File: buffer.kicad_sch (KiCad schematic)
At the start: 3 parts, among them U1 TL072

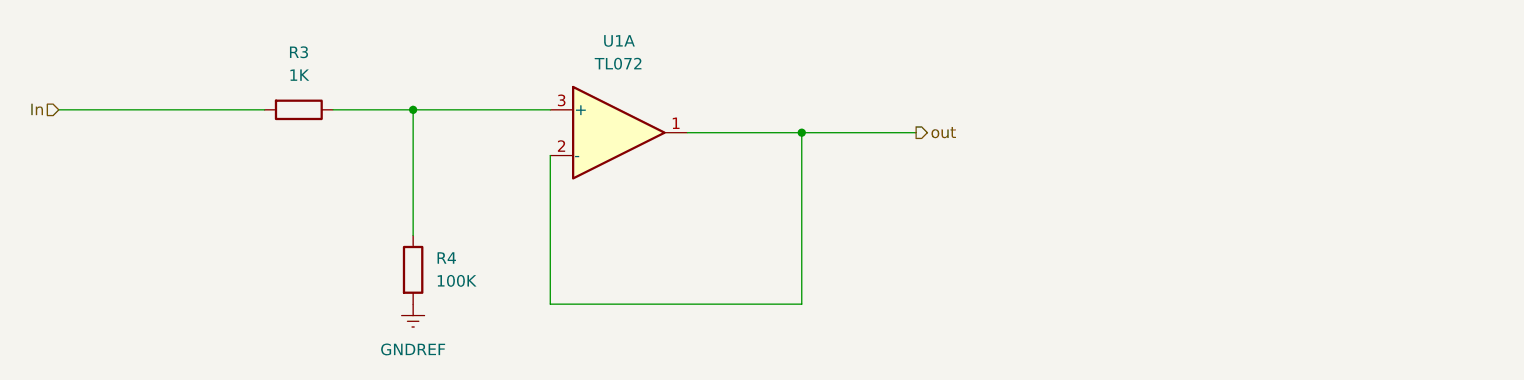
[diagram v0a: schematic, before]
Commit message: Fix input section
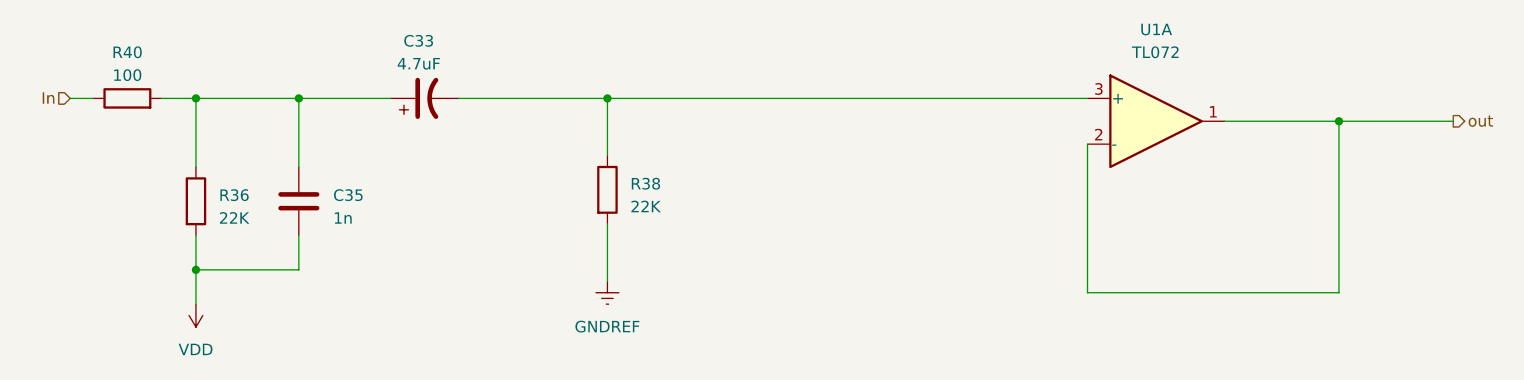
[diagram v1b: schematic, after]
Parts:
- removed R3: 1K, Resistor_THT:R_Axial_DIN0207_L6.3mm_D2.5mm_P7.62mm_Horizontal, symbol Device:R
- removed R4: 100K, Resistor_THT:R_Axial_DIN0207_L6.3mm_D2.5mm_P7.62mm_Horizontal, symbol Device:R
- added C33: 4.7uF, symbol Device:C_Polarized_US
- added C35: 1n, symbol Device:C
- added R36, R38: 22K, symbol Device:R
- added R40: 100, symbol Device:R
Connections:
- net GNDREF: now also R38.2
- net In: now also R40.1
- net at U1.3 (+): now also C33.2, R38.1
- new net: C33.1, C35.1, R36.1, R40.2
- new net VDD: C35.2, R36.2
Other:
- moved on the sheet: U1A
